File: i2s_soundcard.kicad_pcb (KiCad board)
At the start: 4 copper layers, 83.1 x 50 mm, 19 parts, among them J1 Conn_01x08, J2 Conn_01x06, J3 Conn_01x05, J4 Conn_01x11, J5 Conn_01x04, U1 TLV320AIC3104IRHBT, U2 FSA2275UMX, U3 TPA2006D1DRBR, U4 FSA2275UMX, U5 TPA2006D1DRBR, U6 TLV7111830DSER

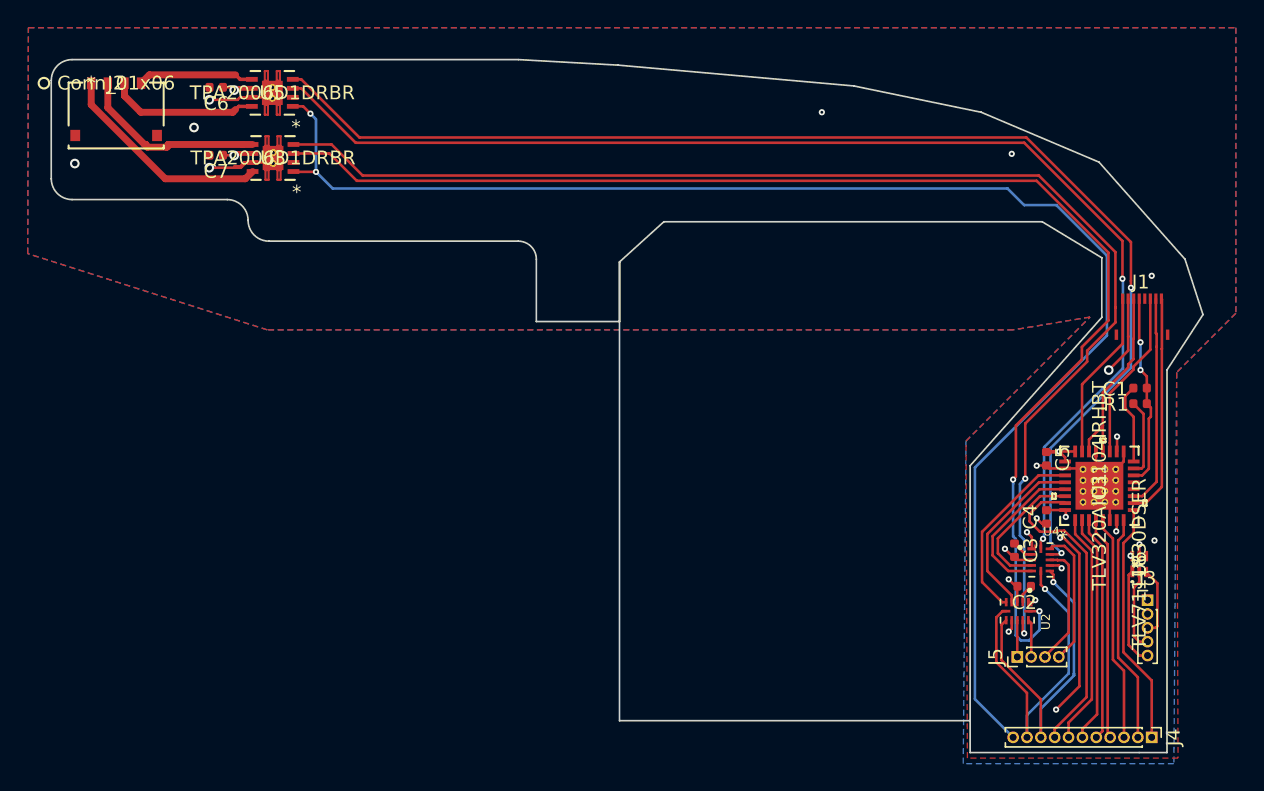
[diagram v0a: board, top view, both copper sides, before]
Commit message: Tweak ground planes a bit.
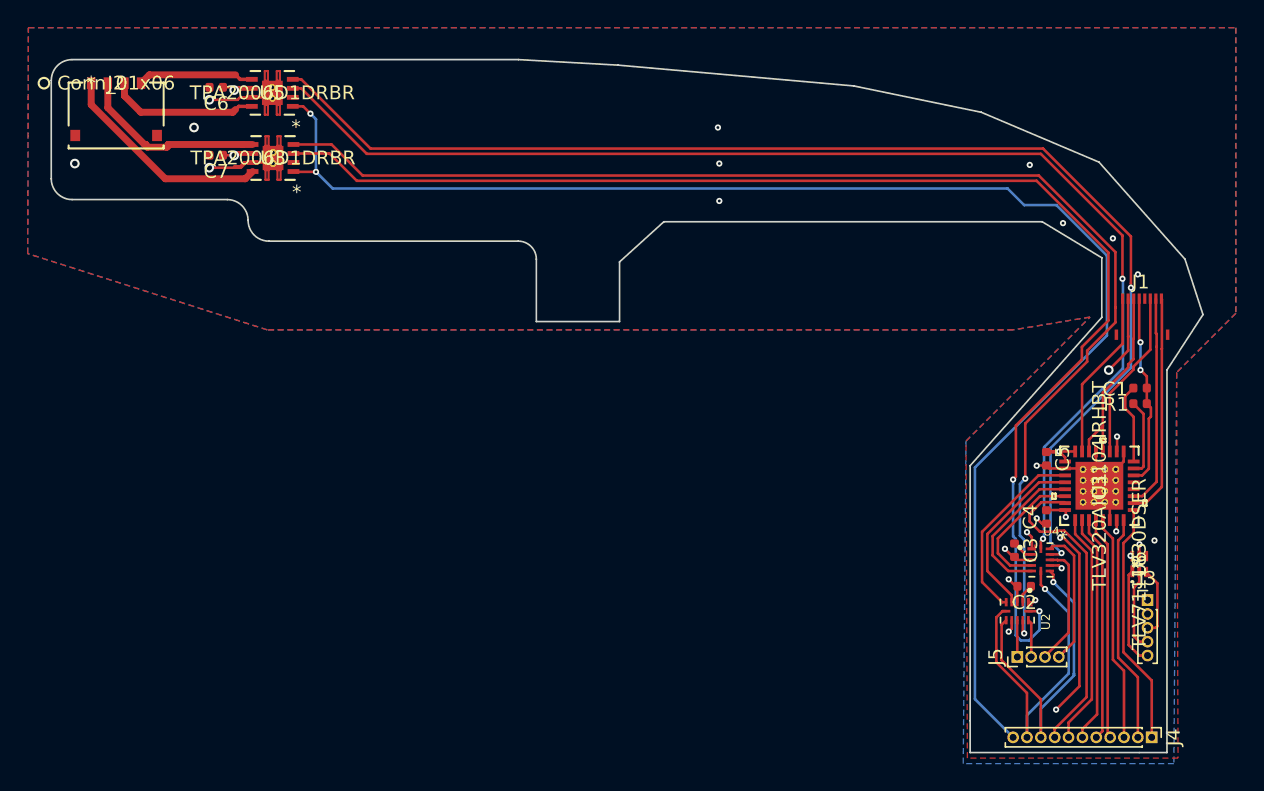
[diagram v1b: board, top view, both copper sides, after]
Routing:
- net GND: vias 16 -> 20
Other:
- outline, holes or cut-outs redrawn
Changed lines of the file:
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@@
   (general
     (thickness 1)
-    (drawings 43)
-    (tracks 420)
+    (drawings 41)
+    (tracks 424)
     (zones 0)
     (modules 19)
@@
   (gr_line (start 166.3 108.3) (end 154.1 108.3) (layer Edge.Cuts) (width 0.12))
   (gr_line (start 122.8 77.2) (end 128.8 77.2) (layer Edge.Cuts) (width 0.12))
-  (gr_line (start 128.8 106) (end 154.1 106) (layer Edge.Cuts) (width 0.12))
   (gr_line (start 163.6 72.6) (end 163.6 76.9) (layer Edge.Cuts) (width 0.12))
   (gr_line (start 163.6 76.9) (end 154.1 87.6) (layer Edge.Cuts) (width 0.12))
@@
   (gr_line (start 159.3 70) (end 132 70) (layer Edge.Cuts) (width 0.12))
   (gr_line (start 132 70) (end 128.8 72.9) (layer Edge.Cuts) (width 0.12))
-  (gr_line (start 128.8 106) (end 128.8 72.9) (layer Edge.Cuts) (width 0.12))
   (gr_text "Round these corners! 1mm radius\n" (at 119 153 90) (layer Cmts.User)
     (effects (font (size 2 2) (thickness 0.15)))
@@
   (via (at 99.2 61.2) (size 0.7) (drill 0.4) (layers F.Cu B.Cu) (net 3))
   (segment (start 99.2 60.315) (end 99.215 60.3) (width 0.19) (layer F.Cu) (net 3))
-  (via (at 143.4 62.1) (size 0.45) (drill 0.2) (layers F.Cu B.Cu) (net 3))
-  (via (at 167.2 73.9) (size 0.45) (drill 0.2) (layers F.Cu B.Cu) (net 3))
+  (via (at 166.2 73.8) (size 0.45) (drill 0.2) (layers F.Cu B.Cu) (net 3))
   (segment (start 159.6 87.585) (end 158.915021 87.585) (width 0.19) (layer F.Cu) (net 3))
   (via (at 158.900021 87.6) (size 0.45) (drill 0.2) (layers F.Cu B.Cu) (net 3))
   (segment (start 158.915021 87.585) (end 158.900021 87.6) (width 0.19) (layer F.Cu) (net 3))
-  (via (at 157.1 65.1) (size 0.45) (drill 0.2) (layers F.Cu B.Cu) (net 3))
   (via (at 167.4 93) (size 0.45) (drill 0.2) (layers F.Cu B.Cu) (net 3))
   (segment (start 157.5 96.315) (end 157.515 96.3) (width 0.19) (layer F.Cu) (net 3))
@@
   (via (at 156.610013 93.6) (size 0.45) (drill 0.2) (layers F.Cu B.Cu) (net 3))
   (segment (start 157.195013 94.185) (end 156.610013 93.6) (width 0.19) (layer F.Cu) (net 3))
+  (via (at 164.4 71.2) (size 0.45) (drill 0.2) (layers F.Cu B.Cu) (net 3))
+  (via (at 136 65.8) (size 0.45) (drill 0.2) (layers F.Cu B.Cu) (net 3))
+  (via (at 135.9 63.2) (size 0.45) (drill 0.2) (layers F.Cu B.Cu) (net 3))
+  (via (at 136 68.5) (size 0.45) (drill 0.2) (layers F.Cu B.Cu) (net 3))
+  (via (at 158.4 65.9) (size 0.45) (drill 0.2) (layers F.Cu B.Cu) (net 3))
+  (via (at 160.8 70.1) (size 0.45) (drill 0.2) (layers F.Cu B.Cu) (net 3))
   (segment (start 157.9 96.885) (end 158.485 96.3) (width 0.19) (layer F.Cu) (net 4))
   (segment (start 157.9 97.45) (end 157.9 96.885) (width 0.19) (layer F.Cu) (net 4))
@@
   (segment (start 158.344801 100.210001) (end 157.755199 100.210001) (width 0.19) (layer B.Cu) (net 27))
   (segment (start 159.1 99.454802) (end 158.344801 100.210001) (width 0.19) (layer B.Cu) (net 27))
-  (segment (start 158.157406 63.91999) (end 165.7 71.462584) (width 0.19) (layer F.Cu) (net 28))
-  (segment (start 165.7 71.462584) (end 165.7 74.270195) (width 0.19) (layer F.Cu) (net 28))
-  (segment (start 105.840001 59.725001) (end 110.03499 63.91999) (width 0.19) (layer F.Cu) (net 28))
-  (segment (start 110.03499 63.91999) (end 158.157406 63.91999) (width 0.19) (layer F.Cu) (net 28))
-  (segment (start 165.7 74.270195) (end 165.7 74.759978) (width 0.19) (layer F.Cu) (net 28))
-  (segment (start 105.225001 59.725001) (end 105.840001 59.725001) (width 0.19) (layer F.Cu) (net 28))
   (via (at 165.7 74.759978) (size 0.45) (drill 0.2) (layers F.Cu B.Cu) (net 28))
   (segment (start 159.85 94) (end 160.600008 94) (width 0.19) (layer F.Cu) (net 28))
@@
   (segment (start 165.7 80.537414) (end 159.9 86.337416) (width 0.19) (layer B.Cu) (net 28))
   (segment (start 159.9 86.337416) (end 159.9 93.11257) (width 0.19) (layer B.Cu) (net 28))
-  (segment (start 165.090013 71.390013) (end 165.090013 74.109987) (width 0.19) (layer F.Cu) (net 29))
-  (segment (start 105.840001 60.374999) (end 109.765002 64.3) (width 0.19) (layer F.Cu) (net 29))
-  (segment (start 109.765002 64.3) (end 158 64.3) (width 0.19) (layer F.Cu) (net 29))
-  (segment (start 158 64.3) (end 165.090013 71.390013) (width 0.19) (layer F.Cu) (net 29))
-  (segment (start 105.225001 60.374999) (end 105.840001 60.374999) (width 0.19) (layer F.Cu) (net 29))
+  (segment (start 110.83499 64.71999) (end 159.357406 64.71999) (width 0.19) (layer F.Cu) (net 28))
+  (segment (start 105.225001 59.725001) (end 105.840001 59.725001) (width 0.19) (layer F.Cu) (net 28))
+  (segment (start 105.840001 59.725001) (end 110.83499 64.71999) (width 0.19) (layer F.Cu) (net 28))
+  (segment (start 165.7 71.062584) (end 165.7 74.44178) (width 0.19) (layer F.Cu) (net 28))
+  (segment (start 159.357406 64.71999) (end 165.7 71.062584) (width 0.19) (layer F.Cu) (net 28))
+  (segment (start 165.7 74.44178) (end 165.7 74.759978) (width 0.19) (layer F.Cu) (net 28))
   (via (at 165.090013 74.109987) (size 0.45) (drill 0.2) (layers F.Cu B.Cu) (net 29))
   (segment (start 159.2 93.032867) (end 159.357847 92.87502) (width 0.19) (layer F.Cu) (net 29))
@@
   (segment (start 165.124999 74.144973) (end 165.124999 80.575001) (width 0.19) (layer B.Cu) (net 29))
   (segment (start 159.434094 86.265906) (end 159.434094 92.798773) (width 0.19) (layer B.Cu) (net 29))
+  (segment (start 165.090013 70.990013) (end 165.090013 74.109987) (width 0.19) (layer F.Cu) (net 29))
+  (segment (start 110.565002 65.1) (end 159.2 65.1) (width 0.19) (layer F.Cu) (net 29))
+  (segment (start 105.840001 60.374999) (end 110.565002 65.1) (width 0.19) (layer F.Cu) (net 29))
+  (segment (start 159.2 65.1) (end 165.090013 70.990013) (width 0.19) (layer F.Cu) (net 29))
+  (segment (start 105.225001 60.374999) (end 105.840001 60.374999) (width 0.19) (layer F.Cu) (net 29))
   (segment (start 159.614559 90.800441) (end 159.6 90.815) (width 0.19) (layer F.Cu) (net 30))
   (segment (start 160.950001 90.800441) (end 159.614559 90.800441) (width 0.19) (layer F.Cu) (net 30))
@@
       (pts
         (xy 173.275 76.6) (xy 169 80.875) (xy 168.5 106.9) (xy 164.5 106.2) (xy 164.3375 94.7375)
-        (xy 166.6 81.2) (xy 166.6 73) (xy 156.198438 72.959375) (xy 103.3875 77.8) (xy 86.1 72.3)
-        (xy 86.15 56) (xy 173.275 56)
+        (xy 166.4 81.2) (xy 168 73.2) (xy 164.4 70.1) (xy 163 73.1) (xy 103.3875 77.8)
+        (xy 86.1 72.3) (xy 86.15 56) (xy 173.275 56)
       )
     )
@@
     (polygon
       (pts
-        (xy 166.3 74.6) (xy 166.3 80.9) (xy 160.2 87) (xy 160.2 90.7) (xy 163 93.5)
-        (xy 163 98.5) (xy 159.5 98.5) (xy 159.5 95.9) (xy 157.7 94.1) (xy 157.7 73.2)
-        (xy 164.9 73.2)
+        (xy 164.4 70.5) (xy 167.8 73.4) (xy 166.3 80.9) (xy 160.2 87) (xy 160.2 90.7)
+        (xy 161.3 93.6) (xy 161.3 95.4) (xy 159.35 95.4) (xy 159.5 95.9) (xy 157.7 94.1)
+        (xy 158.9 85.8) (xy 164.3 80.3) (xy 163.4 73)
       )
     )
